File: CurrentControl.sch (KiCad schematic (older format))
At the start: 8 parts, among them P1 CONN_01X01, P3 Current Control, Q401 BUK9575, U201 LMV358

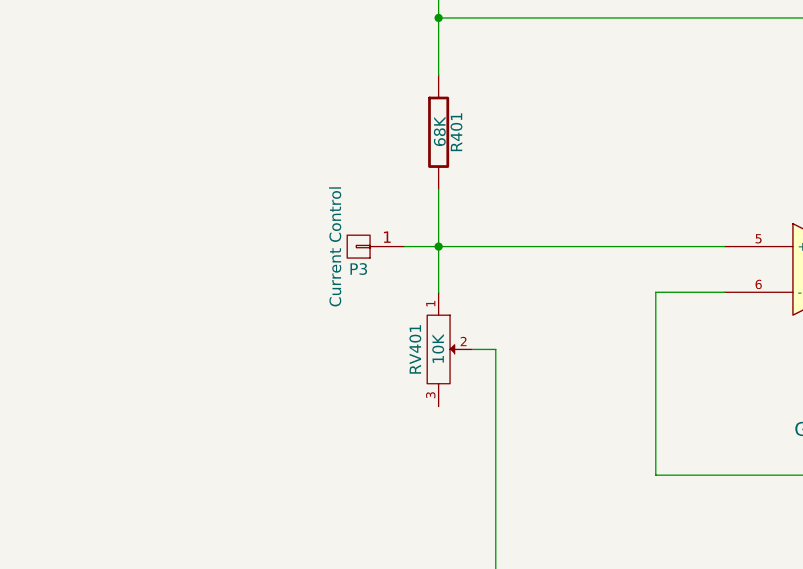
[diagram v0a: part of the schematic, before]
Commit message: Changed footprints, changed layout
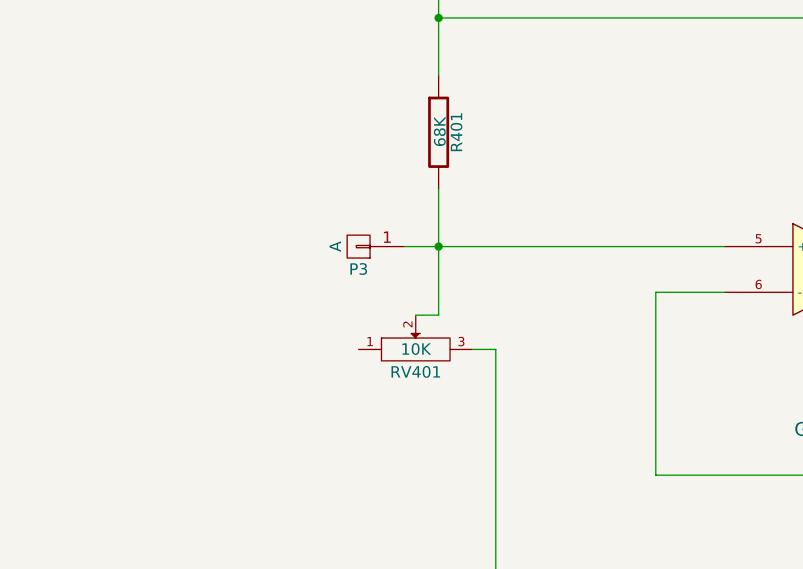
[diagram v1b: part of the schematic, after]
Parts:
- P3: value Current Control -> A; footprint (none) -> Pin_Headers:Pin_Header_Straight_1x01
- R403: footprint Resistors_ThroughHole:Resistor_Horizontal_RM15mm -> Current:1W-Resistor
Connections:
- net Current_Sink-: now also RV401.3; no longer RV401.2
- net at P3.1 (P1), R401.2, U201.5 (+): now also RV401.2; no longer RV401.1
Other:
- moved on the sheet: RV401
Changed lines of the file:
@@
 F 0 "R403" V 8180 5150 50  0000 C CNN
 F 1 ".1" V 8107 5151 50  0000 C CNN
-F 2 "Resistors_ThroughHole:Resistor_Horizontal_RM15mm" V 8030 5150 30  0001 C CNN
+F 2 "Current:1W-Resistor" V 8030 5150 30  0001 C CNN
 F 3 "" H 8100 5150 30  0000 C CNN
 F 4 "AC01000001007JA100" V 8100 5150 60  0001 C CNN "MPN"
@@
 $EndComp
 $Comp
-L GND #PWR7
+L GND #PWR07
 U 1 1 54DADC82
 P 5400 4250
-F 0 "#PWR7" H 5400 4000 60  0001 C CNN
+F 0 "#PWR07" H 5400 4000 60  0001 C CNN
 F 1 "GND" H 5400 4100 60  0000 C CNN
 F 2 "" H 5400 4250 60  0000 C CNN
@@
 L POT RV401
 U 1 1 54DADC9B
-P 3750 4050
-F 0 "RV401" H 3750 3950 50  0000 C CNN
-F 1 "10K" H 3750 4050 50  0000 C CNN
-F 2 "Current:P090L-02F25BR10K" H 3750 4050 60  0001 C CNN
-F 3 "" H 3750 4050 60  0000 C CNN
-F 4 "P090L-02F25BR10K" H 3750 4050 60  0001 C CNN "MPN"
-	1    3750 4050
-	0    1    1    0
+P 3650 4050
+F 0 "RV401" H 3650 3950 50  0000 C CNN
+F 1 "10K" H 3650 4050 50  0000 C CNN
+F 2 "Current:P090L-02F25BR10K" H 3650 4050 60  0001 C CNN
+F 3 "" H 3650 4050 60  0000 C CNN
+F 4 "P090L-02F25BR10K" H 3650 4050 60  0001 C CNN "MPN"
+	1    3650 4050
+	1    0    0    -1
 $EndComp
 Wire Wire Line
@@
 $EndComp
 Wire Wire Line
-	3750 3350 3750 3800
+	3750 3350 3750 3900
 Connection ~ 3750 3600
 Wire Wire Line
@@
 P 3400 3600
 F 0 "P3" H 3400 3700 50  0000 C CNN
-F 1 "Current Control" V 3500 3600 50  0000 C CNN
-F 2 "" H 3400 3600 60  0000 C CNN
+F 1 "A" V 3500 3600 50  0000 C CNN
+F 2 "Pin_Headers:Pin_Header_Straight_1x01" H 3400 3600 60  0001 C CNN
 F 3 "" H 3400 3600 60  0000 C CNN
 	1    3400 3600
 	-1   0    0    1
 $EndComp
+Wire Wire Line
+	3750 3900 3650 3900
 $EndSCHEMATC
